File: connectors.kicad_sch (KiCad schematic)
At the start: 21 parts, among them J10 Serial, J11 Barrel_Jack_Switch, J12 Power, J13 RX In, J14 GND, J15 TX Out, J16 Conn_01x09_Male, J2 Programming, J3 SHIFT0, J4 SHIFT1, J5 PSS, J6 1MHZ, J7 Reset F9T, J8 ANT_VCC, J9 F9T Connector

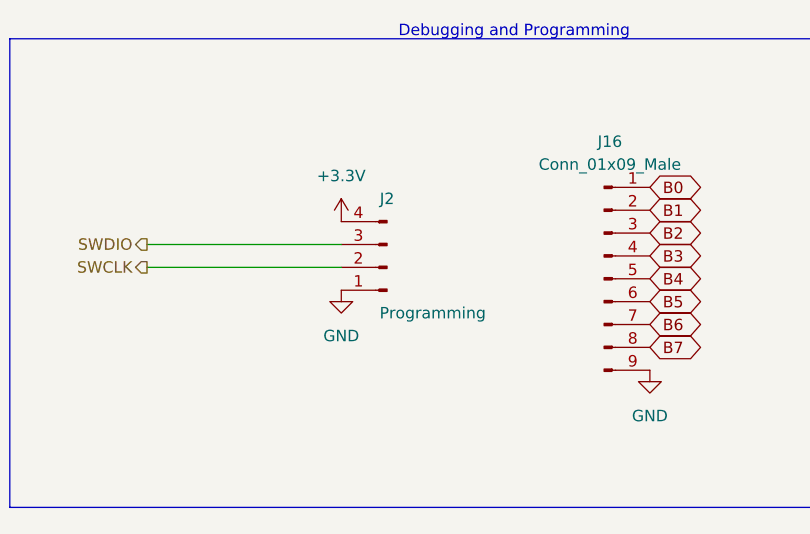
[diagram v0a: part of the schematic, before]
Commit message: Fix inverse numbering of programming header
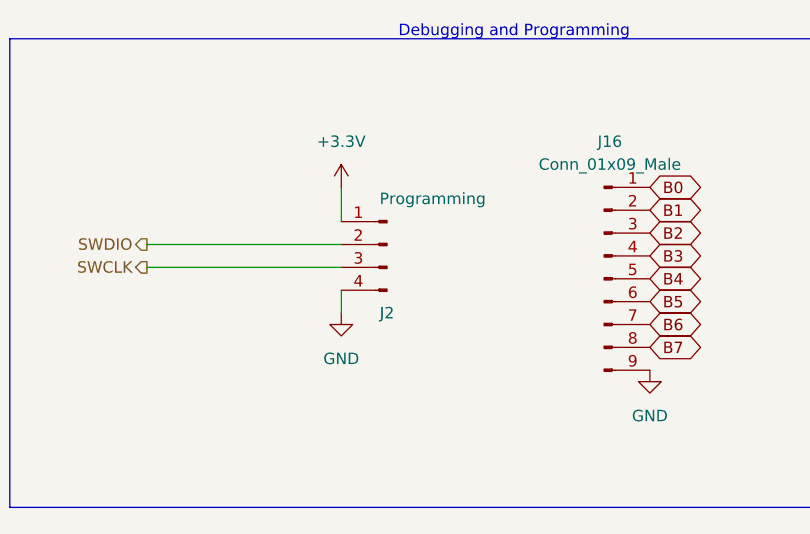
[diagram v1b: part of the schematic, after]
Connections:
- net +3.3V: now also J2.1 (Pin_1); no longer J2.4 (Pin_4)
- net GND: now also J2.4 (Pin_4); no longer J2.1 (Pin_1)
- net SWCLK: now also J2.3 (Pin_3); no longer J2.2 (Pin_2)
- net SWDIO: now also J2.2 (Pin_2); no longer J2.3 (Pin_3)
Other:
- moved on the sheet: J2
